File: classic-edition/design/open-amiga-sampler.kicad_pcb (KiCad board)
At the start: 2 copper layers, 38.1 x 44.5 mm, 18 parts, among them J1 3.5mm stereo phone, J3 DB25_Male, U1 ADC0820CCN, U2 MCP6002-xP^{:3}

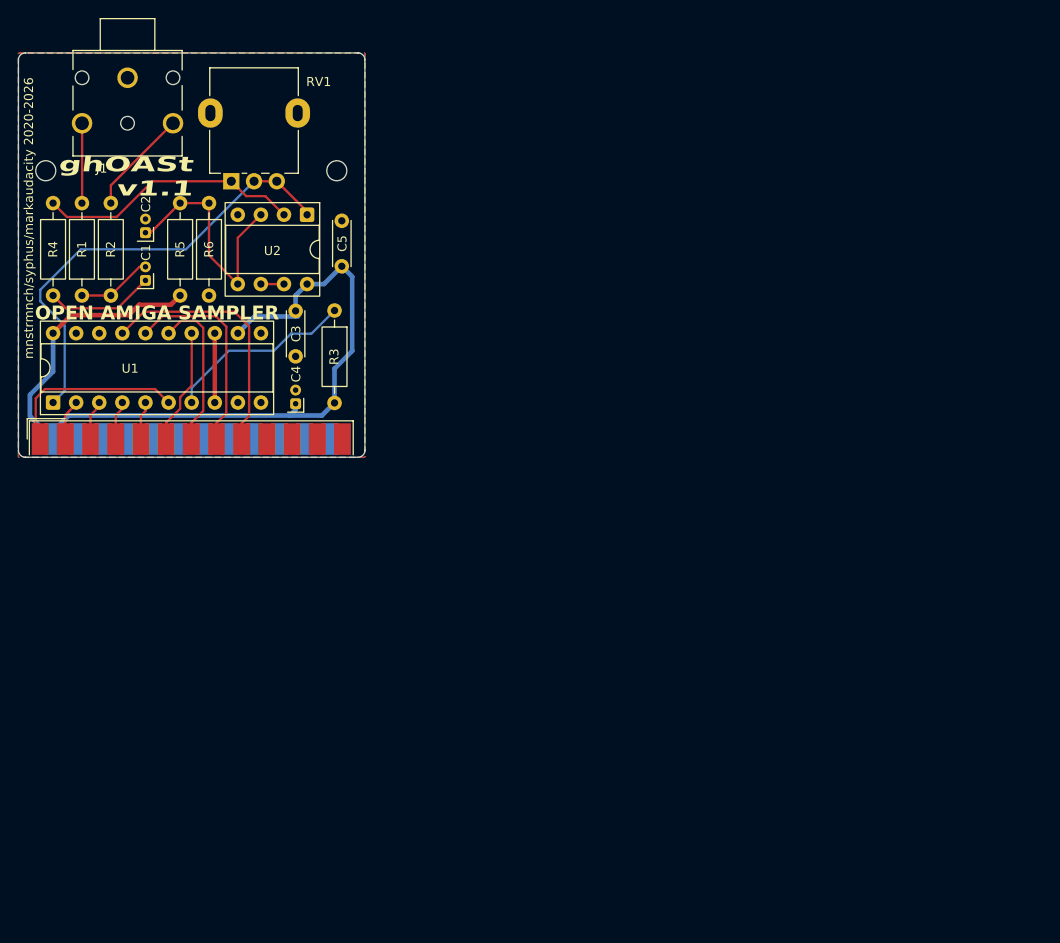
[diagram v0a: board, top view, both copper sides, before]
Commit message: fixing some sync oopsies
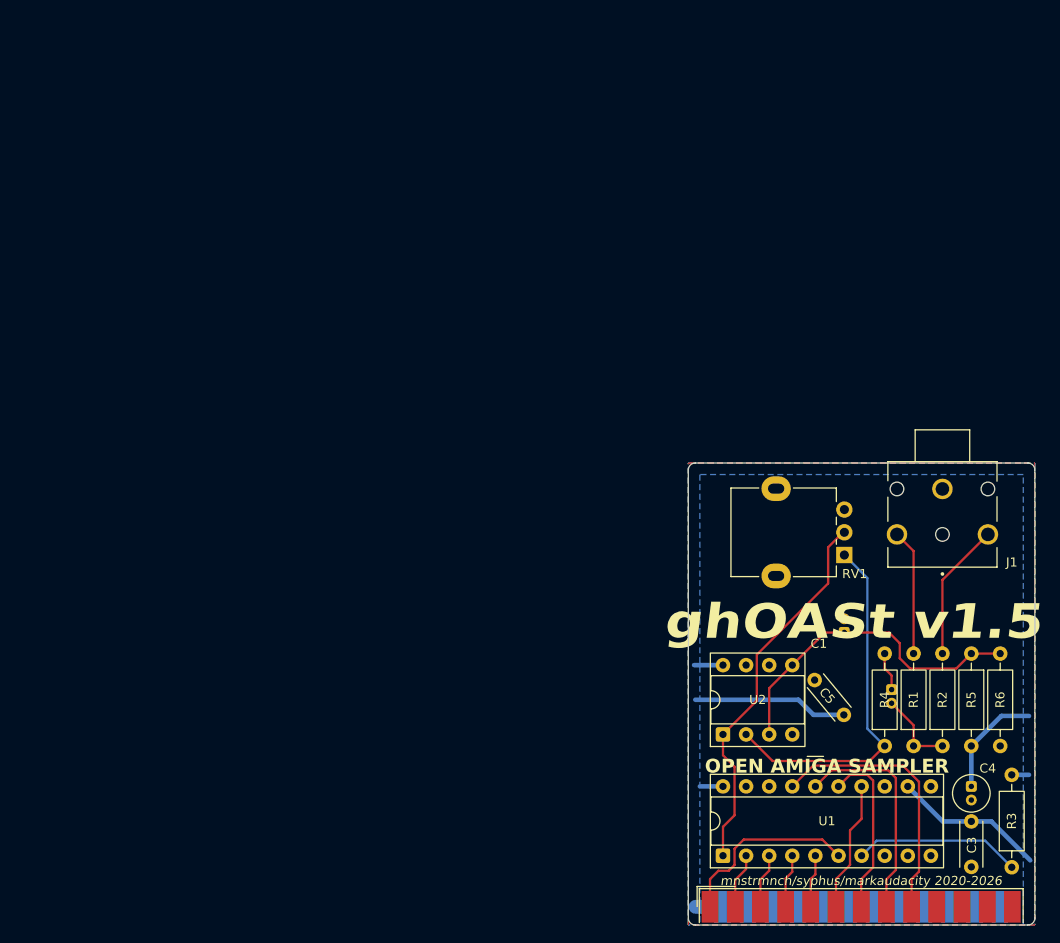
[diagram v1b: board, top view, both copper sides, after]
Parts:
- removed REF** (x2): MountingHole_2.2mm_M2, MountingHole:MountingHole_2.2mm_M2
- moved R4 109.2 mm to (146.2, 93.8), turned to 90 degrees
- moved R2 104.0 mm to (152.6, 93.8)
- moved R1 104.0 mm to (149.4, 93.8)
- moved J1 100.4 mm to (152.6, 65.5)
- moved R6 100.1 mm to (158.9, 93.8)
- moved R5 100.1 mm to (155.8, 83.6)
- moved R3 96.4 mm to (160.2, 107.1), turned to 90 degrees
- moved C1 93.6 mm to (147.0, 87.6), turned to -90 degrees
- moved C3 93.1 mm to (155.8, 102.0)
- moved J3 89.8 mm to (143.7, 111.4)
- moved U1 88.9 mm to (128.5, 105.8)
- moved C2 88.5 mm to (141.8, 81.3)
- moved C4 85.4 mm to (155.8, 98.2), turned to -90 degrees
- moved RV1 78.9 mm to (141.8, 72.8), turned to 180 degrees
- moved C5 74.0 mm to (141.8, 90.3), turned to 130 degrees
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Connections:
- RV1 pad : (no net) -> GND
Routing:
- net VCC: track 96.6 -> 56.7 mm
- net Net-(U2A--): track 29.2 -> 40.0 mm
- net Net-(U2A-+): track 27.2 -> 36.3 mm
- net Net-(C1-~-Pad1): track 12.0 -> 4.18 mm
- net /AD_IN: track 50.0 -> 42.2 mm
- net GND: track 7.67 -> 0.00 mm
- net Net-(J1-PadT): track 8.47 -> 13.7 mm
- net Net-(J1-PadR): track 11.5 -> 15.0 mm
- net Net-(U2B--): track 2.54 -> 0.00 mm
- net Net-(U1-MODE): track 20.8 -> 18.4 mm
- net /D6: track 22.9 -> 24.5 mm
- net /D4: track 12.8 -> 14.4 mm
- net /D0: track 4.51 -> 6.11 mm
- net /D2: track 4.32 -> 5.92 mm
- net /D3: track 4.22 -> 5.83 mm
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- added copper zone on B.Cu, net VCC
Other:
- board size 38.1 x 44.5 mm -> 38.1 x 50.8 mm
- board text added: "ghOASt v1.5"
- board text added: "v1.5"
- board text removed: "C2"
- board text removed: "ghOASt v1.1"
- board text removed: "v1.1"
